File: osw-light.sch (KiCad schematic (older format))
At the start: 53 parts, among them J1 Conn_01x02, Q1 2N7002, SW1 SW_Push, SW2 SW_Push, SW4 SW_Push, SW5 SW_Push, U1 DS3231MZ, U10 XC6209, U11 MCP73831T-2ACI_OT, U13 XC6209, U2 BMA400, U3 BMP280, U4 GC9A01_IPS_display, U5 USB-OTG, U6 CH340E, U7 ttgo-32-micro, U9 TPS2115A

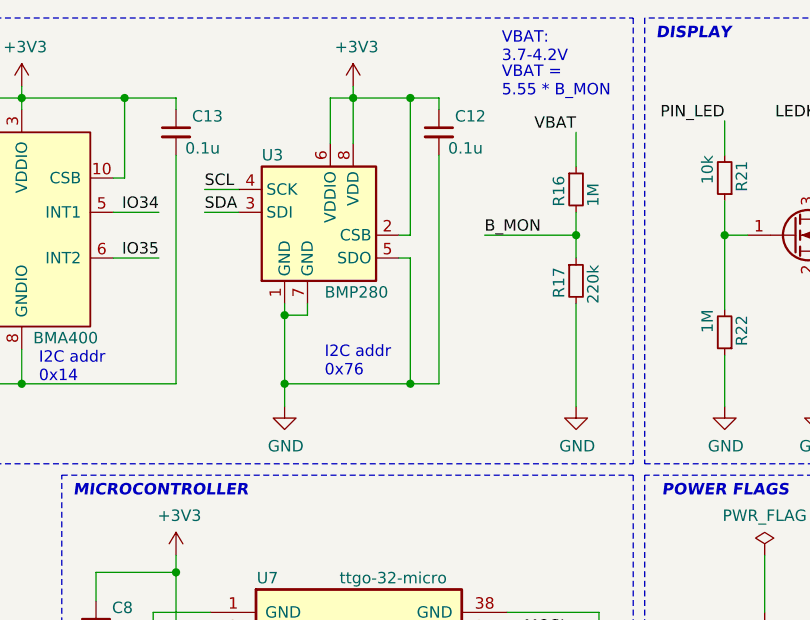
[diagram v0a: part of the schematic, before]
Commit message: rev 3.1, remove bme280, improve layout
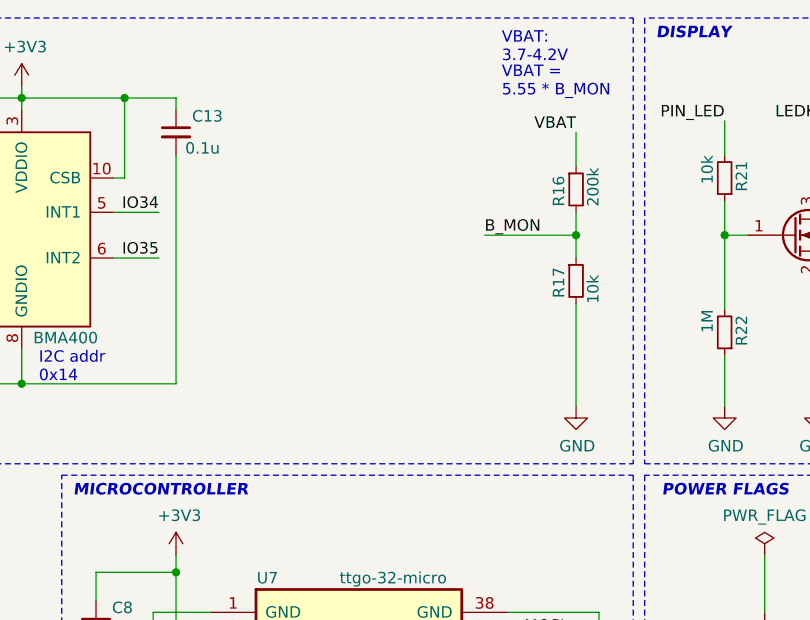
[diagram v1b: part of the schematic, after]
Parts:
- removed C12: 0.1u, Capacitor_SMD:C_0603_1608Metric, symbol Device:C_Small
- removed U3: BMP280, open-Smartwatch:Bosch_LGA-8_2x2.5mm_P0.65mm_ClockwisePinNumbering, symbol open-Smartwatch:BMP280
- R16: value 1M -> 200k
- R17: value 220k -> 10k
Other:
- note removed: "I2C addr\n0x76"
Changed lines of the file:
@@
 Sheet 1 1
 Title "Open-Smartwatch-Light"
-Date "2020-11-18"
-Rev "3.0"
+Date "2021-01-03"
+Rev "3.1"
 Comp ""
 Comment1 ""
@@
 	1    0    0    1
 $EndComp
-Wire Wire Line
-	4175 1800 4175 1750
-Wire Wire Line
-	4375 800  4375 850
-$Comp
-L power:+3V3 #PWR06
-U 1 1 5F71770B
-P 4375 800
-F 0 "#PWR06" H 4375 650 50  0001 C CNN
-F 1 "+3V3" H 4390 973 50  0000 C CNN
-F 2 "" H 4375 800 50  0001 C CNN
-F 3 "" H 4375 800 50  0001 C CNN
-	1    4375 800
-	1    0    0    -1
-$EndComp
-$Comp
-L open-Smartwatch:BMP280 U3
-U 1 1 5F716A88
-P 4275 1450
-F 0 "U3" H 3975 1800 50  0000 L CNN
-F 1 "BMP280" H 4250 1200 50  0000 L CNN
-F 2 "open-Smartwatch:Bosch_LGA-8_2x2.5mm_P0.65mm_ClockwisePinNumbering" H 4275 750 50  0001 C CNN
-F 3 "https://ae-bst.resource.bosch.com/media/_tech/media/datasheets/BST-BMP280-DS001.pdf" H 4275 1450 50  0001 C CNN
-	1    4275 1450
-	1    0    0    -1
-$EndComp
 NoConn ~ 10350 3000
 NoConn ~ 8550 3900
@@
 NoConn ~ 700  1650
 NoConn ~ 1700 1250
-Text Label 3725 1250 0    50   ~ 0
-SCL
-Wire Wire Line
-	3725 1250 3875 1250
-Text Label 3725 1350 0    50   ~ 0
-SDA
-Wire Wire Line
-	3725 1350 3875 1350
-Wire Wire Line
-	4075 2200 4075 2100
-$Comp
-L power:GND #PWR010
-U 1 1 5F72B249
-P 4075 2200
-F 0 "#PWR010" H 4075 1950 50  0001 C CNN
-F 1 "GND" H 4080 2027 50  0000 C CNN
-F 2 "" H 4075 2200 50  0001 C CNN
-F 3 "" H 4075 2200 50  0001 C CNN
-	1    4075 2200
-	1    0    0    -1
-$EndComp
-Wire Wire Line
-	4075 1800 4175 1800
-Connection ~ 4075 1800
-Wire Wire Line
-	4075 1800 4075 1750
 $Comp
 L Connector_Generic:Conn_01x02 J1
@@
 P 5350 1250
 F 0 "R16" V 5275 1175 50  0000 L CNN
-F 1 "1M" V 5425 1175 50  0000 L CNN
+F 1 "200k" V 5425 1175 50  0000 L CNN
 F 2 "Resistor_SMD:R_0603_1608Metric" H 5350 1250 50  0001 C CNN
 F 3 "~" H 5350 1250 50  0001 C CNN
@@
 P 5350 1650
 F 0 "R17" V 5275 1575 50  0000 L CNN
-F 1 "220k" V 5425 1550 50  0000 L CNN
+F 1 "10k" V 5425 1550 50  0000 L CNN
 F 2 "Resistor_SMD:R_0603_1608Metric" H 5350 1650 50  0001 C CNN
 F 3 "~" H 5350 1650 50  0001 C CNN
@@
 Text Label 3850 5350 0    50   ~ 0
 BTN2
-Text Label 3400 4000 0    50   ~ 0
-B_MON
 Wire Wire Line
 	3750 4400 3400 4400
@@
 $EndComp
 $Comp
-L Device:C_Small C12
-U 1 1 5F828FE0
-P 4750 1000
-F 0 "C12" H 4820 1070 50  0000 L CNN
-F 1 "0.1u" H 4790 930 50  0000 L CNN
-F 2 "Capacitor_SMD:C_0603_1608Metric" H 4750 1000 50  0001 C CNN
-F 3 "~" H 4750 1000 50  0001 C CNN
-	1    4750 1000
-	1    0    0    -1
-$EndComp
-$Comp
 L Device:C_Small C13
 U 1 1 5F8293A4
@@
 Wire Wire Line
 	3375 1200 3325 1200
-Wire Wire Line
-	4625 1450 4575 1450
-Wire Wire Line
-	4575 1550 4625 1550
-Text Notes 4250 2075 0    50   ~ 0
-I2C addr\n0x76
 Text Notes 1350 2075 0    50   ~ 0
 I2C addr\n0x68
 Text Notes 3000 2100 0    50   ~ 0
 I2C addr\n0x14
-Wire Wire Line
-	4625 1550 4625 2100
-Wire Wire Line
-	3400 4000 3750 4000
 Wire Wire Line
 	4150 5250 4150 5050
@@
 	2725 2100 2725 2200
 Wire Wire Line
-	4075 2100 4625 2100
-Connection ~ 4075 2100
-Wire Wire Line
-	4075 2100 4075 1800
-Connection ~ 4625 2100
-Wire Wire Line
-	4375 850  4625 850
-Wire Wire Line
-	4750 850  4750 900
-Connection ~ 4375 850
-Wire Wire Line
-	4375 850  4375 1050
-Wire Wire Line
-	4275 850  4375 850
-Wire Wire Line
-	4275 850  4275 1050
-Wire Wire Line
-	4625 850  4625 1450
-Connection ~ 4625 850
-Wire Wire Line
-	4625 850  4750 850
-Wire Wire Line
-	4750 1100 4750 2100
-Wire Wire Line
-	4625 2100 4750 2100
-Wire Wire Line
 	3600 2925 3250 2925
 Wire Wire Line
@@
 Wire Wire Line
 	3600 2925 3600 2850
-Wire Wire Line
-	3750 3100 3500 3100
-Wire Wire Line
-	3500 3100 3500 3350
-Wire Wire Line
-	3500 3350 3250 3350
 Wire Wire Line
 	3250 3350 3250 3250
@@
 	8200 4525 11100 4525
 NoConn ~ 3750 3500
-NoConn ~ 3750 3400
 $Comp
 L Device:R_Small R21
@@
 Wire Wire Line
 	2250 1600 2325 1600
+Wire Wire Line
+	3400 4000 3750 4000
+NoConn ~ 3750 3400
+Wire Wire Line
+	3500 3350 3250 3350
+Wire Wire Line
+	3750 3100 3500 3100
+Wire Wire Line
+	3500 3100 3500 3350
+Text Label 3400 4000 0    50   ~ 0
+B_MON
 $EndSCHEMATC

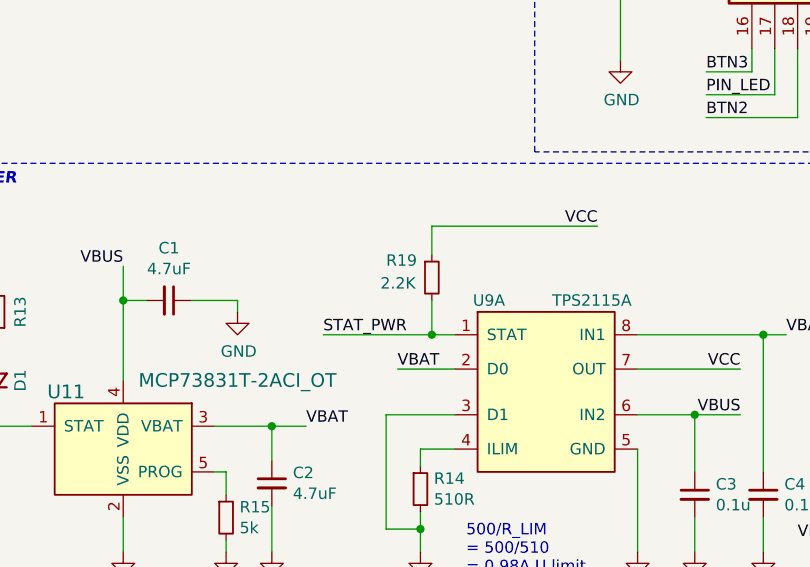
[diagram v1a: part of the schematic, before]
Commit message: rev 3.2: set R19 to 220k - improve standby from 2mA to 0.35mA
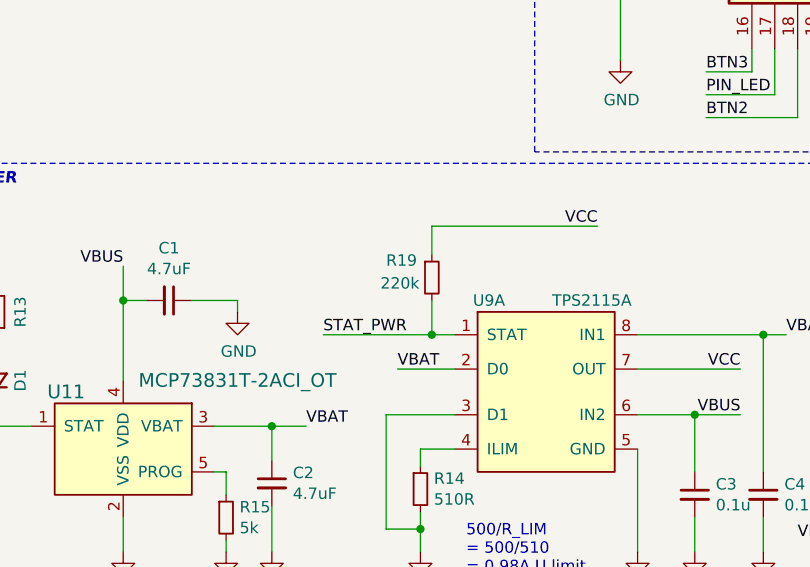
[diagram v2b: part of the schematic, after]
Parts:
- R19: value 2.2K -> 220k
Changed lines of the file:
@@
 Sheet 1 1
 Title "Open-Smartwatch-Light"
-Date "2021-01-03"
-Rev "3.1"
+Date "2021-01-17"
+Rev "3.2"
 Comp ""
 Comment1 ""
@@
 P 2650 6050
 F 0 "R19" H 2450 6125 50  0000 L CNN
-F 1 "2.2K" H 2425 6025 50  0000 L CNN
+F 1 "220k" H 2425 6025 50  0000 L CNN
 F 2 "Resistor_SMD:R_0603_1608Metric" H 2650 6050 50  0001 C CNN
 F 3 "~" H 2650 6050 50  0001 C CNN
